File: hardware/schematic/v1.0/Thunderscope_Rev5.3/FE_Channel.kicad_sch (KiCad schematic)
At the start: 105 parts, among them J3_4 UFL, J4_4 UFL, J6 Conn_Coaxial, K1000_4 G6K-2F-RF, K1001_4 G6K-2F-RF, Q1002_4 DMN62D0UW, Q1003_4 DMN62D0UW, U1001_4 TMUX4053, U1008_4 LMH6518, U1009_4 BUF802, U1011_4 OPA140AIDBVR

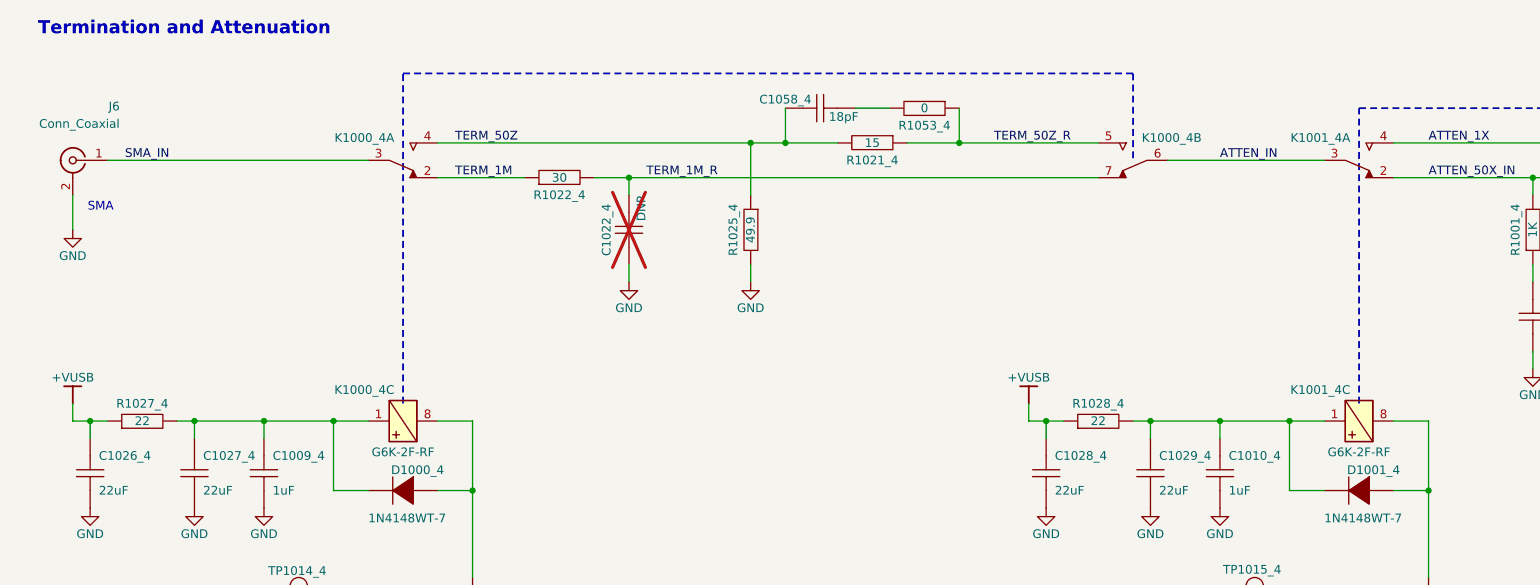
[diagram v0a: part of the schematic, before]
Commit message: sch update
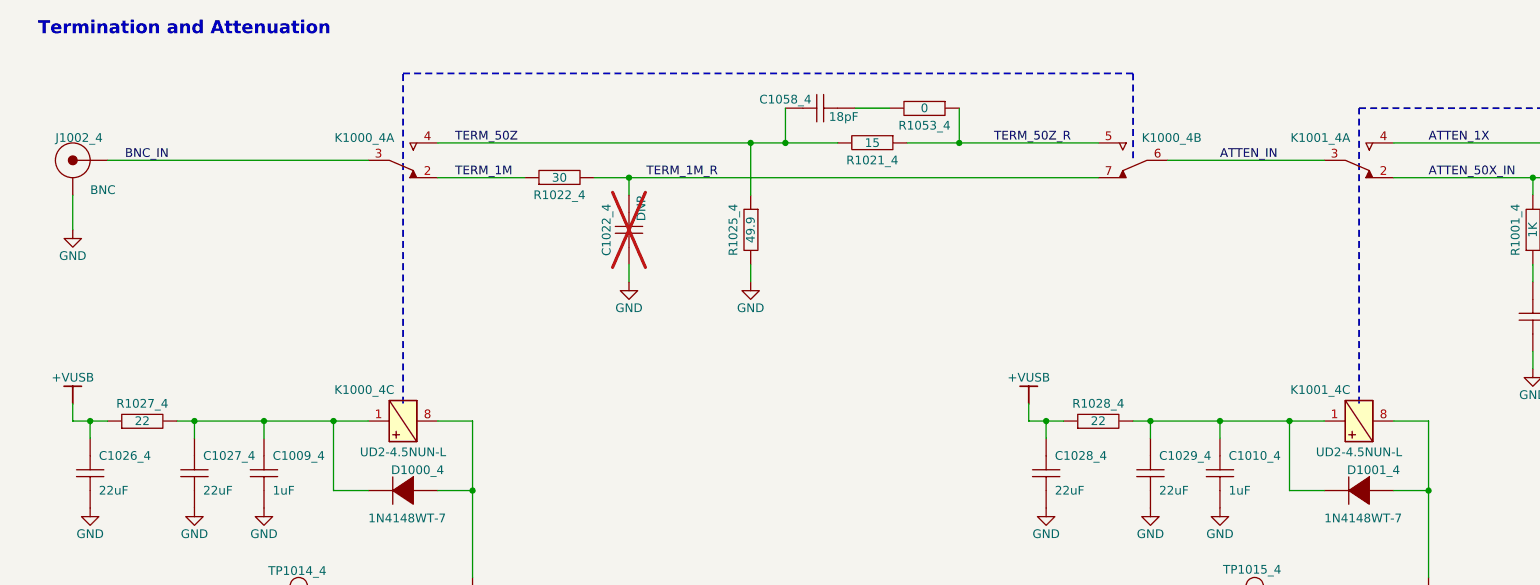
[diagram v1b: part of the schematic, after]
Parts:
- removed J6: Conn_Coaxial, Connector_Coaxial:SMA_Molex_73251-2120_EdgeMount_Horizontal, symbol Connector:Conn_Coaxial
- added J1002_4: BNC, Thunderscope_Rev5:MOL_0731000105, symbol Thunderscope_Rev5:BNC JACK R/A
- K1000_4, K1001_4: value G6K-2F-RF -> UD2-4.5NUN-L
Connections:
- net GND: now also J1002_4.2 (SHIELD)
- net SMA_IN renamed BNC_IN
- net BNC_IN: now also J1002_4.1 (Signal)
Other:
- note removed: "SMA"

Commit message: sch update
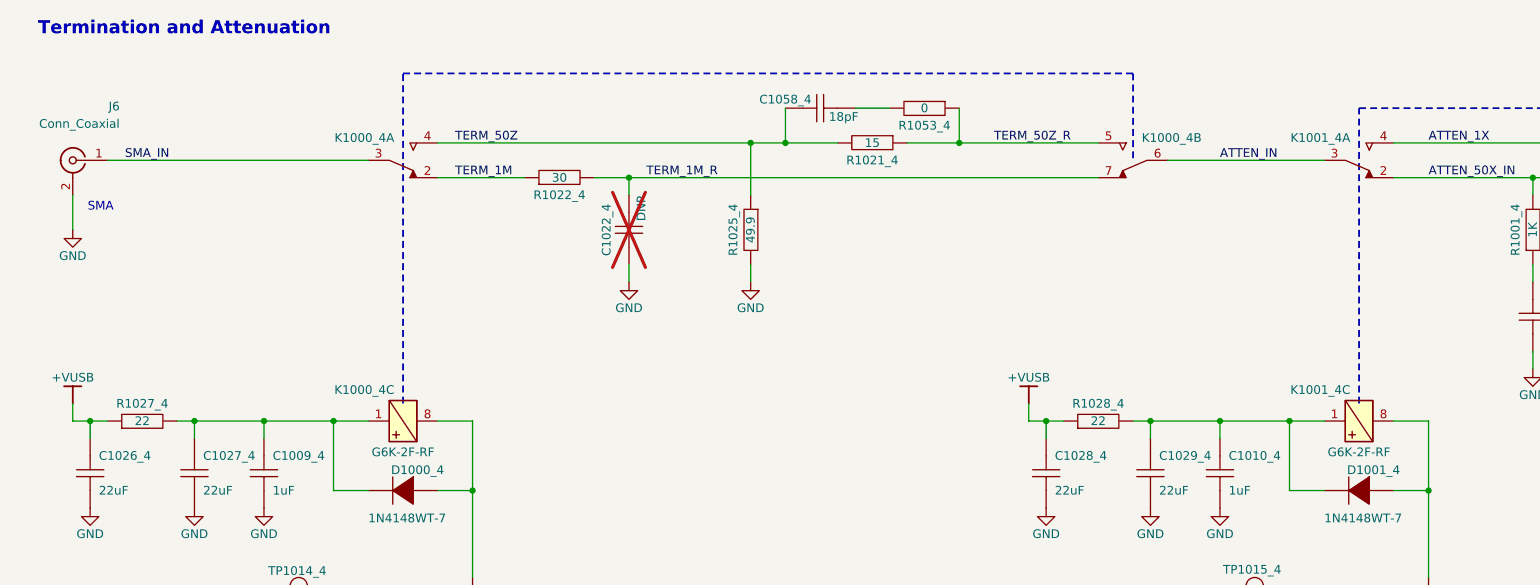
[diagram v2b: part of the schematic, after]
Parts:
- removed J1002_4: BNC, Thunderscope_Rev5:MOL_0731000105, symbol Thunderscope_Rev5:BNC JACK R/A
- added J6: Conn_Coaxial, Connector_Coaxial:SMA_Molex_73251-2120_EdgeMount_Horizontal, symbol Connector:Conn_Coaxial
- K1000_4, K1001_4: value UD2-4.5NUN-L -> G6K-2F-RF
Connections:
- net GND: now also J6.2 (Ext)
- net BNC_IN renamed SMA_IN
- net SMA_IN: now also J6.1 (In)
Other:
- note added: "SMA"
